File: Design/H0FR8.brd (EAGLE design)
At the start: 60 x 60.6 mm, 45 parts, among them Q1 MMBT3904LT1, U1 STM32G0B1CEU6QFN_B1CEU6_STM-L, U2 T2035H-6GD2PAK_T2550_STM-M, U3 VOT8121AM-VT, U4 TLP184_GR-TPL,SE, U5 V275LA4P, X1 XTALL_CSTCE8M00G52

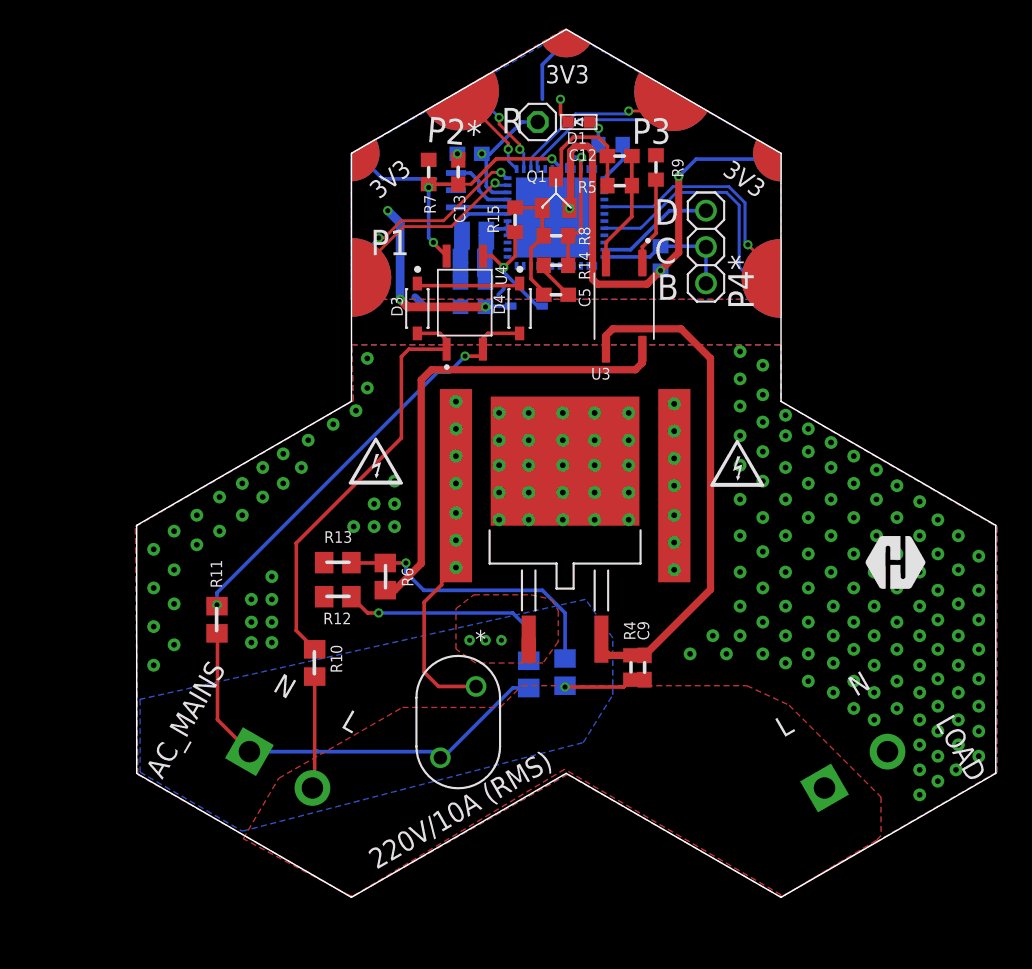
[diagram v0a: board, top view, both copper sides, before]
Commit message: -The final design, all done.
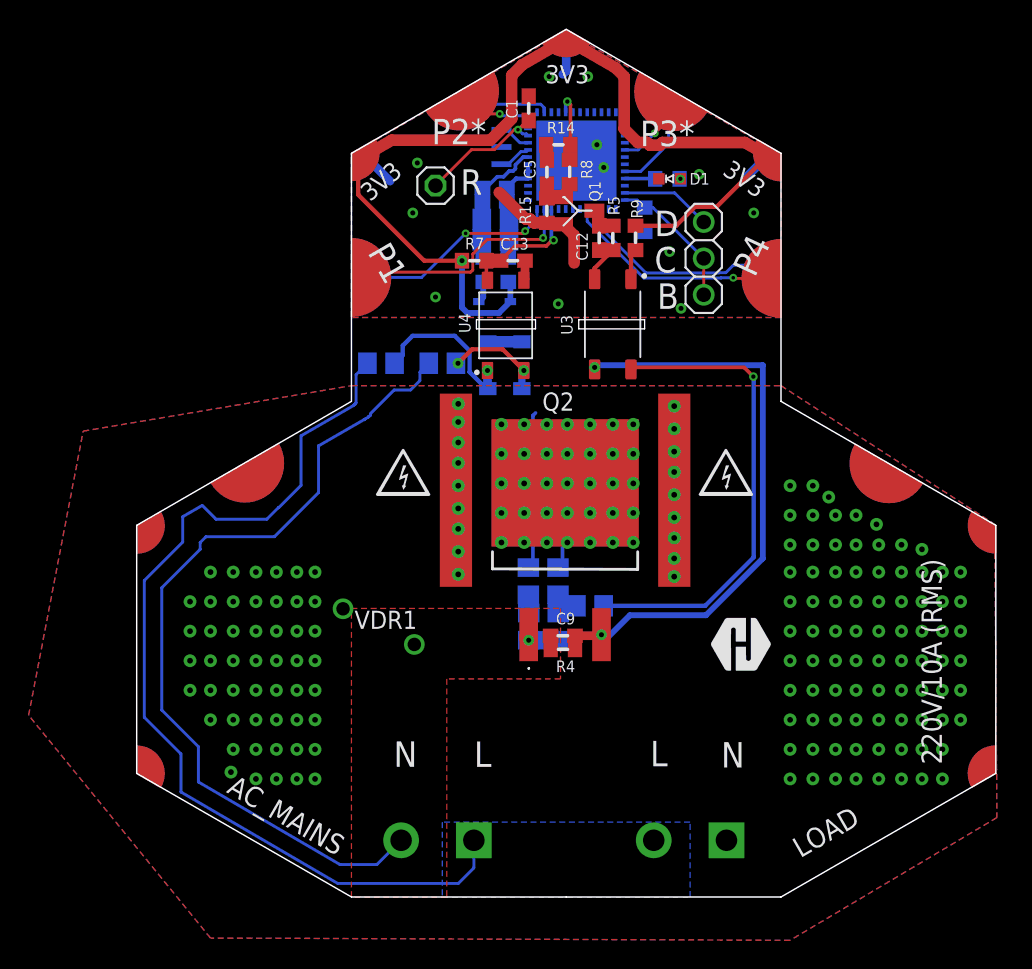
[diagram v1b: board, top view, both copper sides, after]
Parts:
- removed D3, D4: STMICROELECTRONICS_BAT46ZFILMSTMICROELECTRONICS_BAT46ZFILM_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, HEXABITZ_RCLS:STMICROELECTRONICS_BAT46ZFILM_3
- removed U2: T2035H-6GD2PAK_T2550_STM-M, HEXABITZ_ICs:D2PAK_T2550_STM-M
- removed U5: V275LA4P, HEXABITZ_RCLS:LA_07MM_LOW_LTF
- added Q2: T2035H-6G, HEXABITZ_ICs:T2035H6G
- added VDR1: V275LA4P, HEXABITZ_RCLS:LA_07MM_LOW_LTF
- added Z1, Z2: MMSZ5225BT1G, HEXABITZ_RCLS:SOD3716X135N
- C2, C3: device HEXABITZ_RCLS:C-0603-POL -> HEXABITZ_RCLS:C-0805-POL
- D1: device Hexabitz:VLMS1300-GS08 -> HEXABITZ_USER_INTERFACE_PARTS:VLMS1300-GS08
- moved R11 23.8 mm to (-8.57, 28.7), flipped to the bottom, turned to 0 degrees
- moved R10 21.4 mm to (-12.9, 28.7), flipped to the bottom, turned to 0 degrees
- moved R13 15.4 mm to (-0.50, 13.5), flipped to the bottom, turned to 90 degrees
- moved R6 14.5 mm to (1.74, 11.8), flipped to the bottom, turned to 0 degrees
- moved R12 13.4 mm to (-2.56, 13.5), flipped to the bottom, turned to 90 degrees
- moved LOAD 12.6 mm to (8.73, -4.60), turned to 180 degrees
- moved TRIMBLE-LOGO2 12.2 mm to (12.3, 7.23)
- moved AC_MAINS 12.0 mm to (-8.91, -4.60), turned to 180 degrees
- moved C5 8.60 mm to (-1.27, 42.1), turned to 90 degrees
- moved R14 8.42 mm to (-0.48, 44.0)
- moved R 8.41 mm to (-9.05, 41.1)
- moved D1 7.49 mm to (7.30, 41.6)
- moved C13 7.27 mm to (-3.65, 35.9), turned to 0 degrees
- moved R7 6.96 mm to (-6.35, 35.9), turned to 0 degrees
- moved C9 6.13 mm to (-0.16, 9.68), turned to 180 degrees
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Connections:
- removed net N$14: D3.1, D4.1
- removed net USART4_RX: U$1.PAD_PD3, U1.12
- removed net USART4_TX: U$1.PAD_PU3, U1.11
- new net N$12: Z1.2, Z2.2
- net A2: now also LOAD.1, Q2.2, VDR1.2; no longer LOAD.2, U2.2, U5.2
- net AC_MAINS_L: now also AC_MAINS.1, LOAD.2; no longer AC_MAINS.2, LOAD.1
- net AC_MAINS_N: now also AC_MAINS.2, Q2.1, VDR1.1; no longer AC_MAINS.1, U2.1, U5.1
- net LED_INDICATOR: now also U1.33; no longer U1.25
- net N$15: now also Z1.1; no longer D3.2
- net N$16: now also Z2.1; no longer D4.2
- net TRIAC_G: now also Q2.3; no longer U2.3
- net TRIAC_TRIGGER: now also U1.17; no longer U1.20
- net USART1_RX: now also U$1.PAD_PD2; no longer U$1.PAD_PD8
- net USART1_TX: now also U$1.PAD_PU2; no longer U$1.PAD_PU8
- net USART5_RX: now also U$1.PAD_PD8
- net USART5_TX: now also U$1.PAD_PU8
- net USART6_RX: now also U$1.PAD_PD3, U1.48; no longer U$1.PAD_PD2, U1.16
- net USART6_TX: now also U$1.PAD_PU3, U1.47; no longer U$1.PAD_PU2, U1.15
- net ZC_DETECT: now also U1.46; no longer U1.19
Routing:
- net AC_MAINS_L: track 7.85 -> 66.9 mm
- net VDD: track 14.5 -> 71.8 mm, vias 3 -> 1
- net GND: track 61.1 -> 20.7 mm, vias 6 -> 12
- net AC_MAINS_N: track 37.7 -> 60.9 mm, vias 4 -> 1
- net N$16: track 30.3 -> 7.31 mm
- net N$15: track 30.3 -> 11.5 mm, vias 0 -> 1
- net N$7: track 19.9 -> 2.69 mm, vias 1 -> 0
- net USART5_TX: track 0.00 -> 15.4 mm, vias 0 -> 1
- net USART5_RX: track 0.00 -> 15.3 mm
- net USART4_RX: track 14.3 -> 0.00 mm, vias 2 -> 0
- net N$4: track 15.5 -> 1.28 mm, vias 1 -> 0
- net USART4_TX: track 13.3 -> 0.00 mm, vias 1 -> 0
- net USART1_TX: track 16.9 -> 5.28 mm
- net USART1_RX: track 17.7 -> 6.88 mm
- net N$14: track 7.44 -> 0.00 mm
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- added copper zone on layer 16, net AC_MAINS_L
- added copper zone on layer 1, net GND
- removed copper zone on layer 1, net AC_MAINS_L
- removed copper zone on layer 16, net AC_MAINS_N
- removed copper zone on layer 1, net VDD
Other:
- outline, holes or cut-outs redrawn
- board text added: "P3*"
- board text added: "P4"
- board text removed: "P3"
- board text removed: "P4*"
